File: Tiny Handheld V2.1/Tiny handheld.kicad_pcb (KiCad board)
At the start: 2 copper layers, 34.3 x 58.4 mm, 44 parts, among them IC1 BQ21040DBVR, J1 VDisplay/prog1, J2 HDisplay/prog, J3 USB_C_Receptacle_USB2.0, U1 ATtiny85-20P, U2 ATtiny85-20S

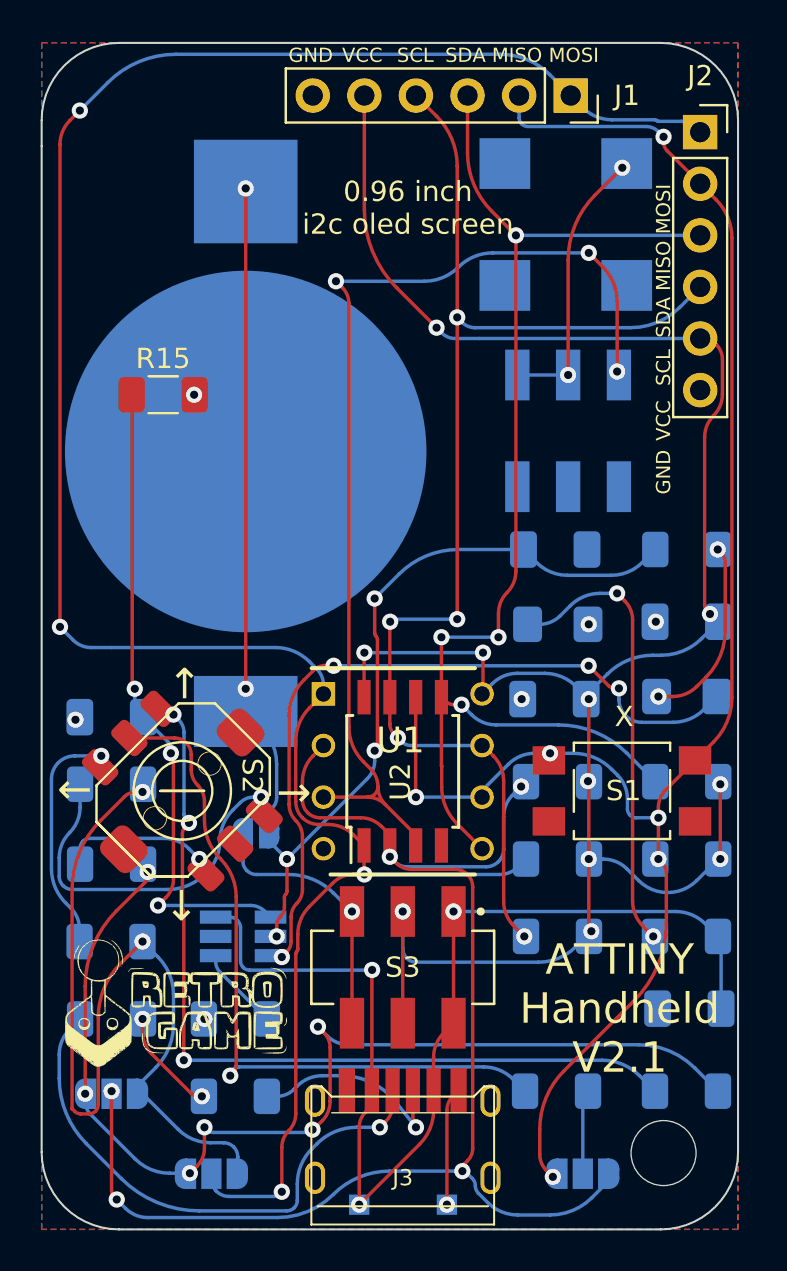
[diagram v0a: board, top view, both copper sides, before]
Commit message: cleanup
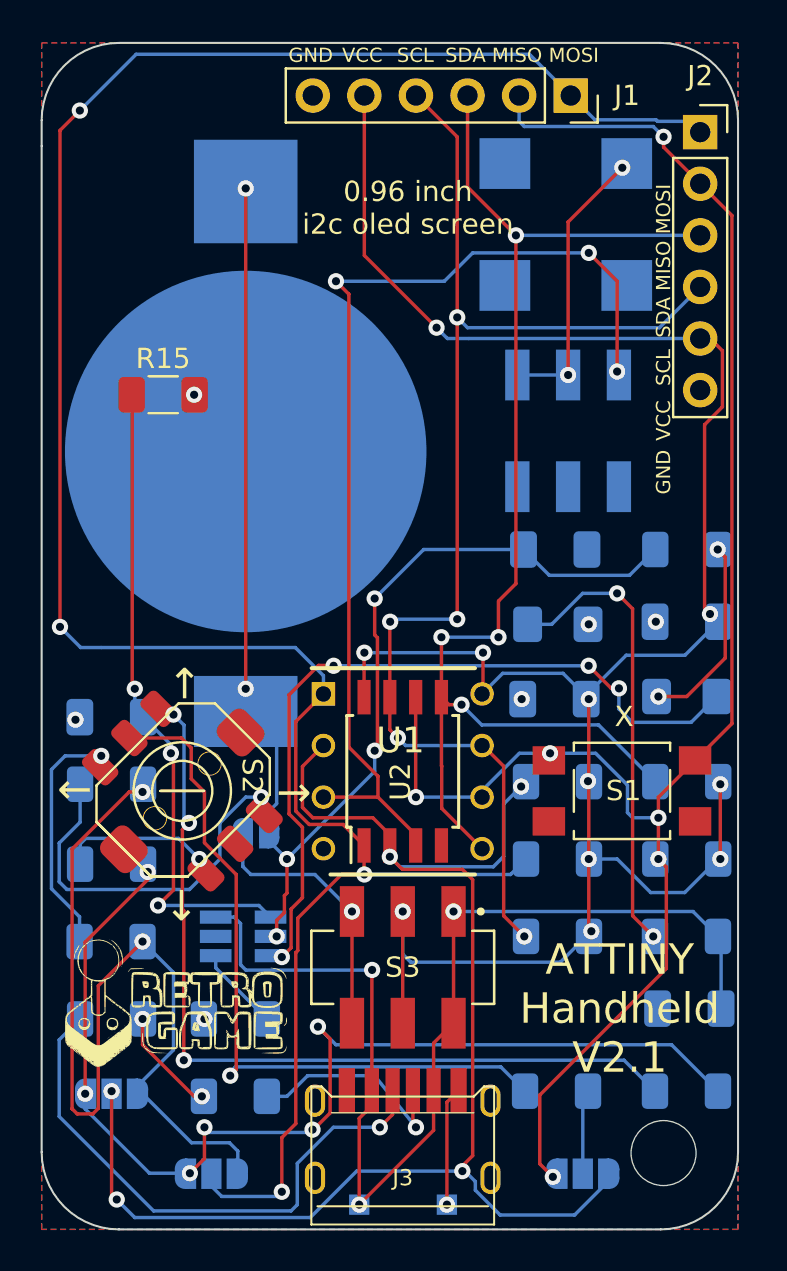
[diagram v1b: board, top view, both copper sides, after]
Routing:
- net PB5/RES: track 114.8 -> 116.4 mm
- net VCC: track 104.4 -> 105.9 mm
- net PB3: track 70.4 -> 71.9 mm
- net PB1/MISO: track 84.4 -> 85.9 mm
- net Net-(JP1-Pad1): track 43.0 -> 44.1 mm
- net Net-(J3-PadA5): track 27.0 -> 27.9 mm
- net Net-(JP1-Pad3): track 53.3 -> 54.2 mm
- net PB2/SCL/SCK: track 63.1 -> 63.9 mm
- net PB0/SDA/MOSI: track 62.6 -> 63.4 mm
- net Net-(D2-Pad1): track 36.9 -> 37.5 mm
- net Net-(C6-Pad1): track 35.6 -> 36.3 mm
- net Net-(R7-Pad2): track 17.7 -> 18.3 mm
- net Net-(R5-Pad2): track 35.1 -> 35.7 mm
- net PB4: track 52.1 -> 51.5 mm
- net ExtVCC: track 54.0 -> 54.6 mm
